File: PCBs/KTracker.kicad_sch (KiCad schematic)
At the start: 40 parts, among them J1 Conn_01x02_Female, J2 Conn_01x04_Female, P1 USB_C_Plug_USB2.0, SW1 Option/FLASH Switch, SW3 SW_SPDT MAIN POWER, U1 ME6211C, U2 TP4056, U6 ESP-12F, U7 CH340C, U9 MPU-9250

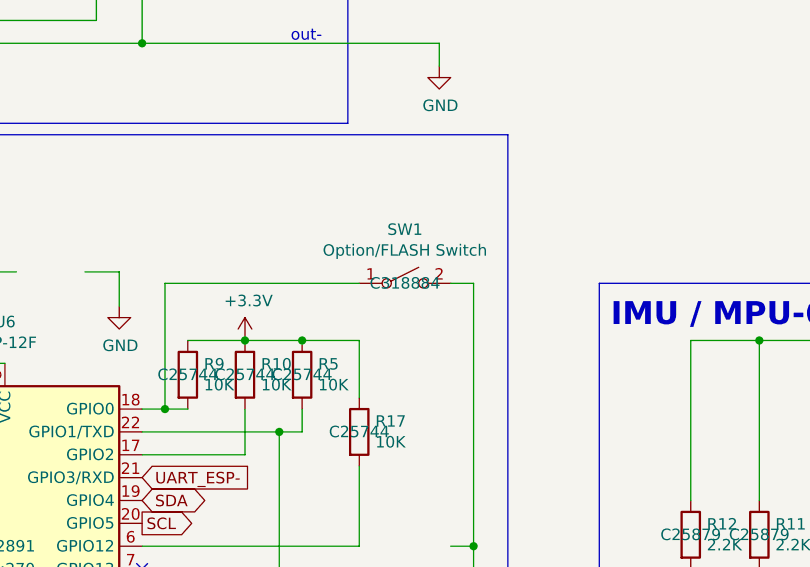
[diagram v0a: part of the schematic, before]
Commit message: clear silk
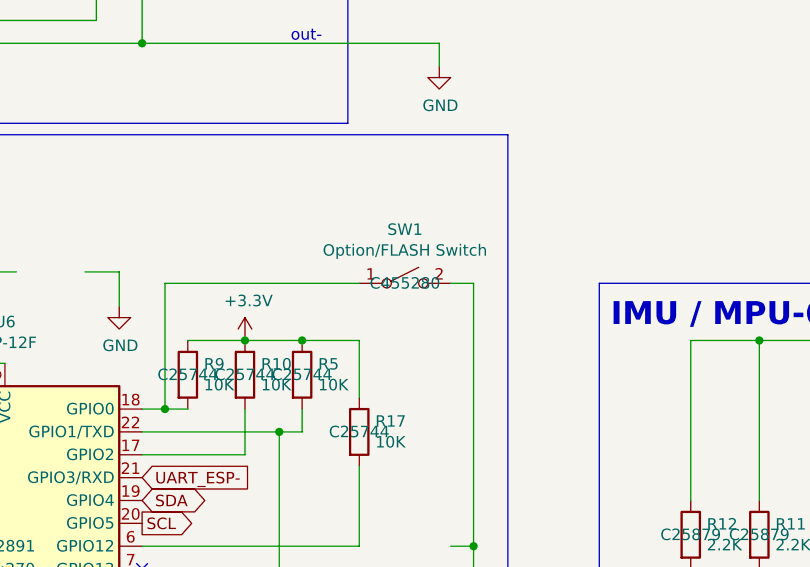
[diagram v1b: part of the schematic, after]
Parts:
- SW1: LCSC C318884 -> C455280
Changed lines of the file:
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@@
       (effects (font (size 1.27 1.27)) hide)
     )
-    (property "LCSC" "C318884" (id 4) (at 163.83 97.79 0))
+    (property "LCSC" "C455280" (id 4) (at 163.83 97.79 0))
     (pin "1")
     (pin "2")

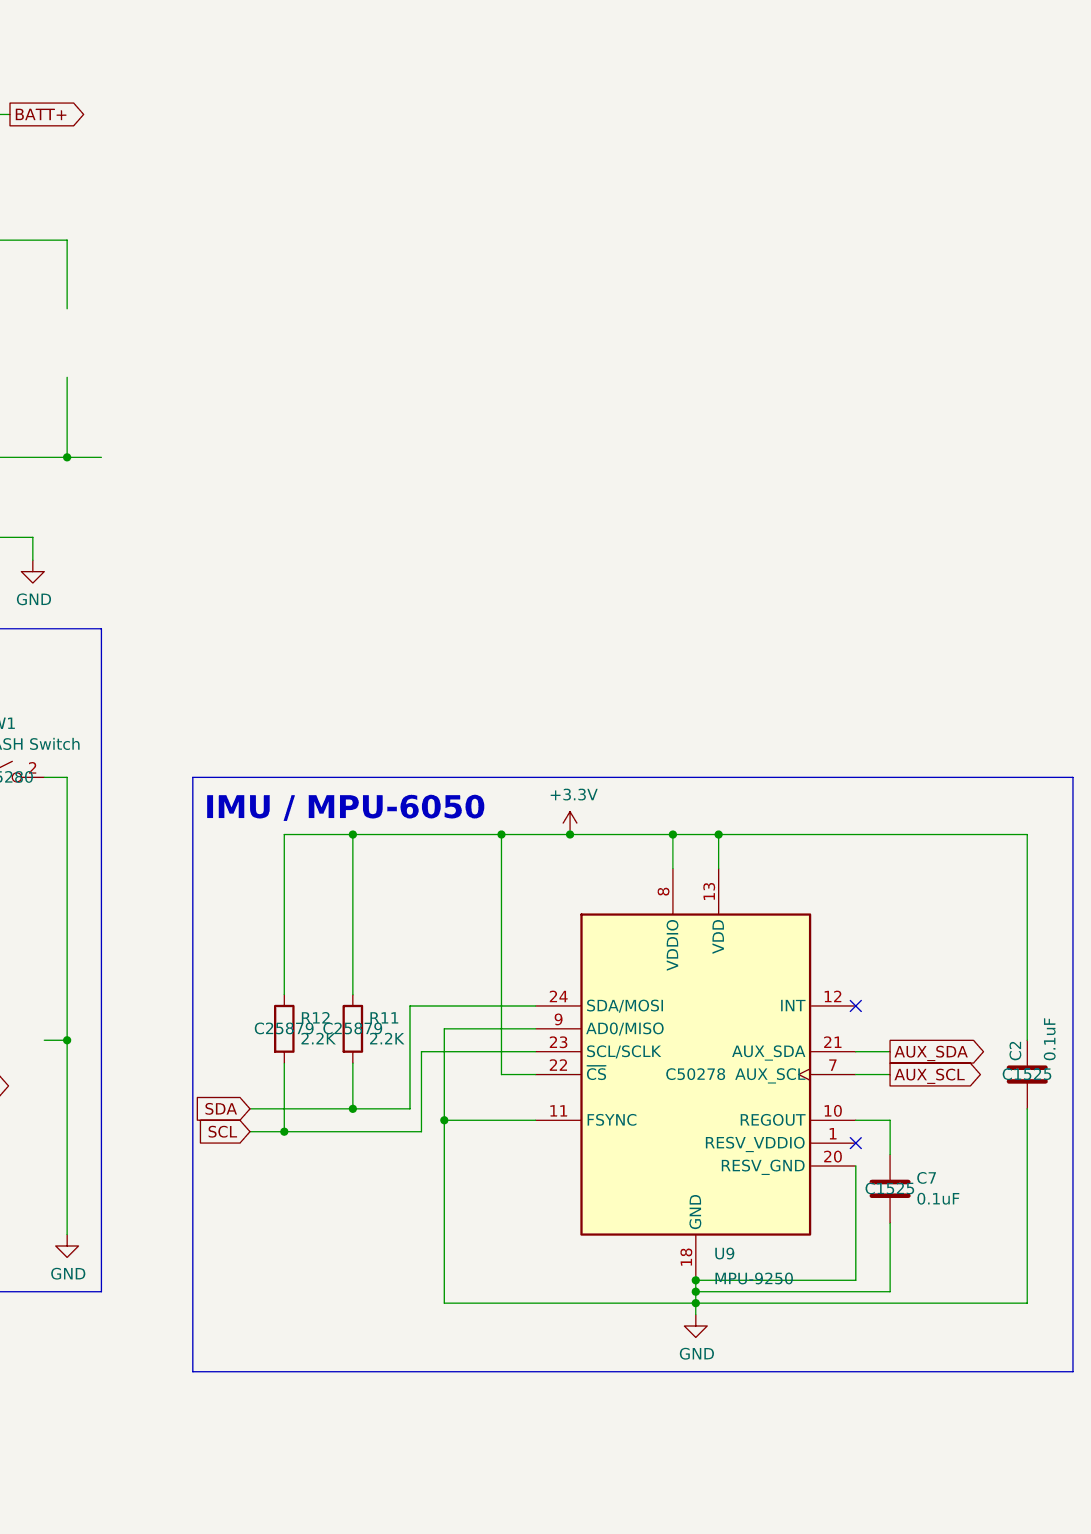
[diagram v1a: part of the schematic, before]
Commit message: yay
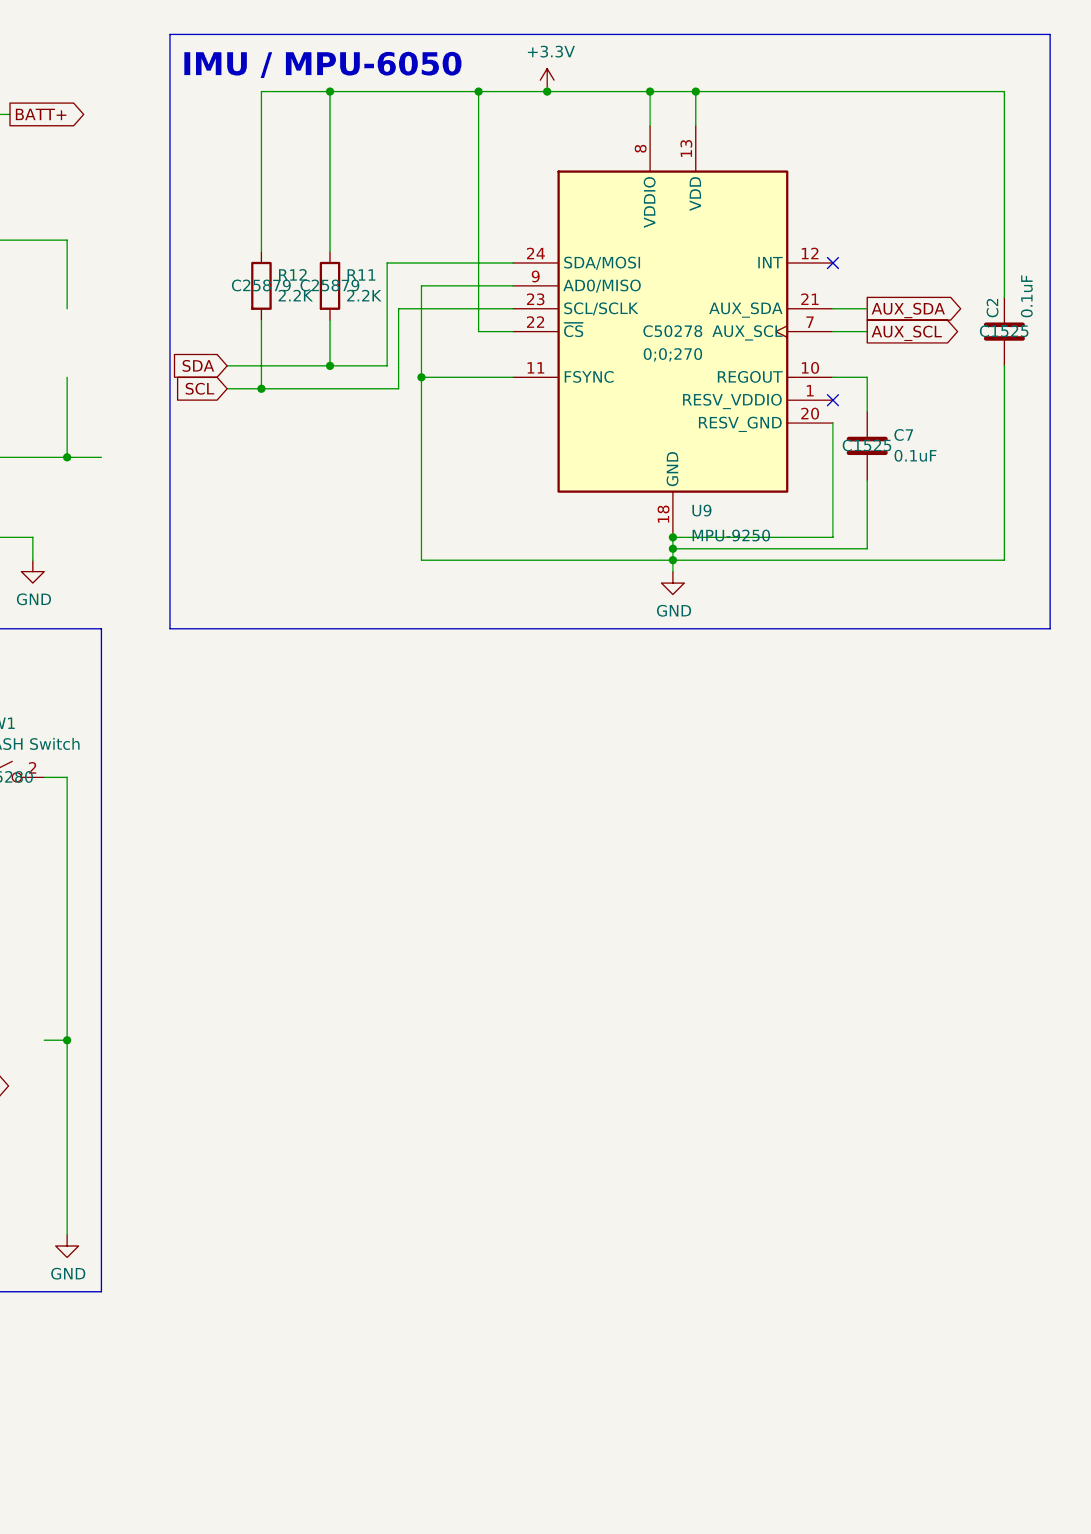
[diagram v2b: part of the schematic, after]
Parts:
- U9: JLCPCB_CORRECTION (none) -> 0;0;270
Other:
- company: github.com/Kamilake/KamiTrack-SlimeVR-PCB -> github.com/Kamilake/KTracker-SlimeVR-PCB
- title: KamiTrack-SlimeVR-PCB -> KTracker-SlimeVR-PCB
- moved on the sheet: C2, C7, R11, R12, U9
